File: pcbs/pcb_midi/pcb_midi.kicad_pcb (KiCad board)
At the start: 2 copper layers, 12 parts, among them J1 DIN_IN, J2 DIN_OUT, J3 RXTX, U1 6N137, U2 74AHCT125

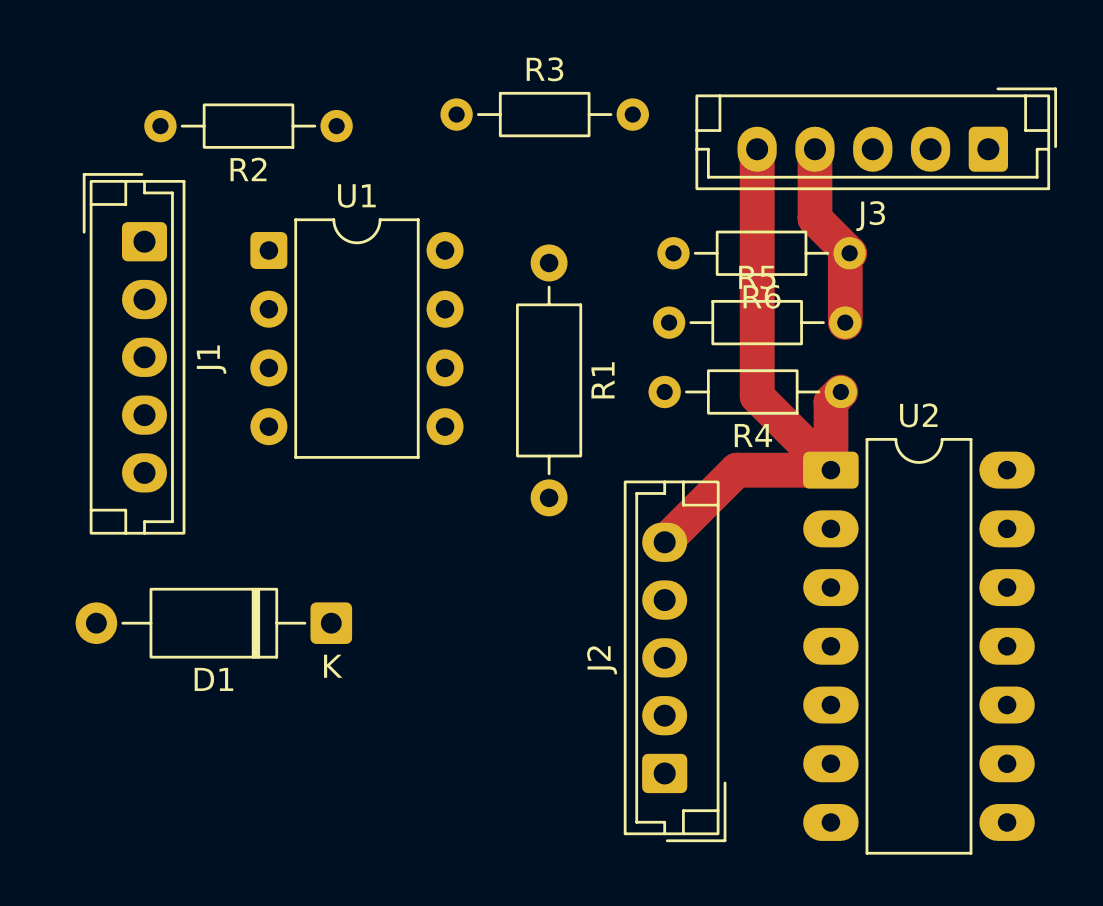
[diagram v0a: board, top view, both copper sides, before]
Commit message: pcb:midi wip
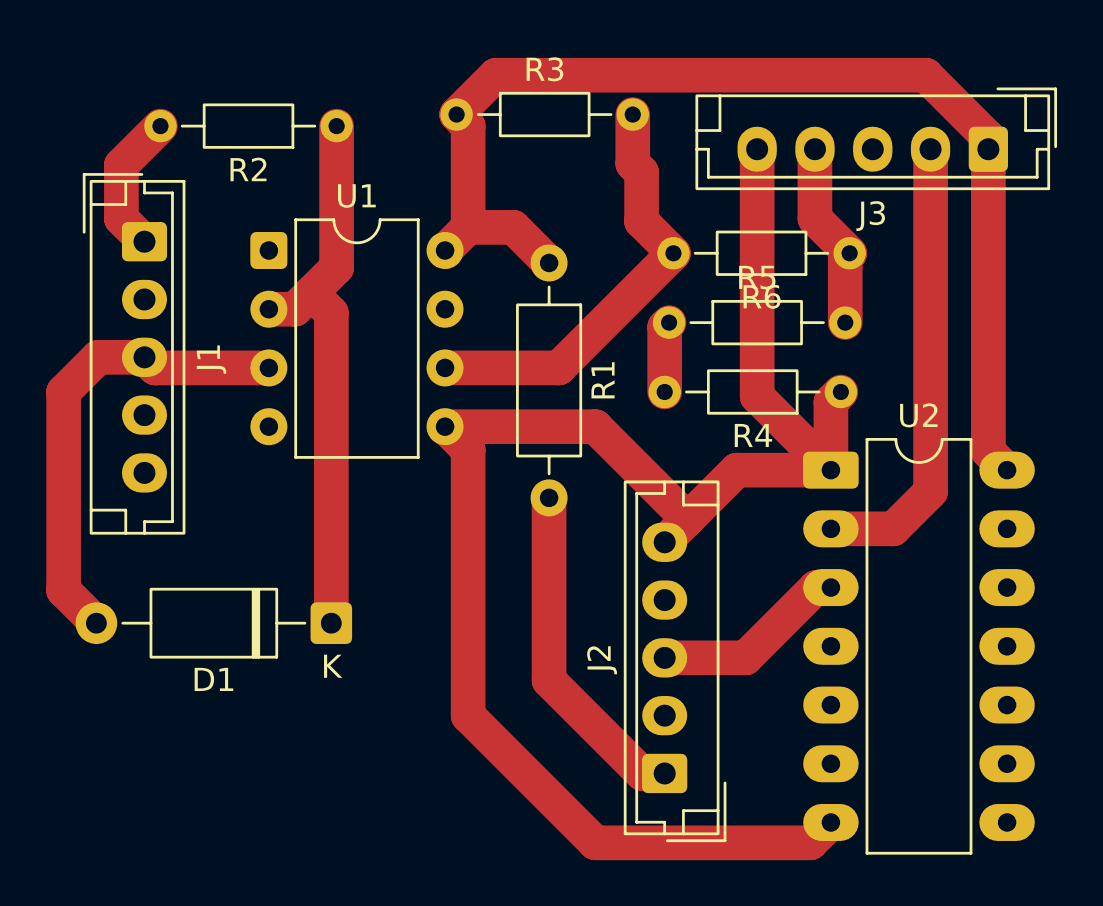
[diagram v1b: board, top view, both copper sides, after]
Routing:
- net +5V: track 0.00 -> 50.2 mm
- net GND: track 27.2 -> 70.6 mm
- net Net-(D1-K): track 0.00 -> 24.4 mm
- net Net-(D1-A): track 0.00 -> 20.3 mm
- net TX: track 0.00 -> 19.8 mm
- net Net-(U1-VO): track 0.00 -> 18.7 mm
- net Net-(J2-Pin_1): track 0.00 -> 14.6 mm
- net Net-(J2-Pin_3): track 0.00 -> 8.45 mm
- net Net-(J1-Pin_1): track 0.00 -> 6.11 mm
- net Net-(R4-Pad2): track 0.00 -> 3.08 mm
